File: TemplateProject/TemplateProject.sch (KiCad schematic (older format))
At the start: 0 parts

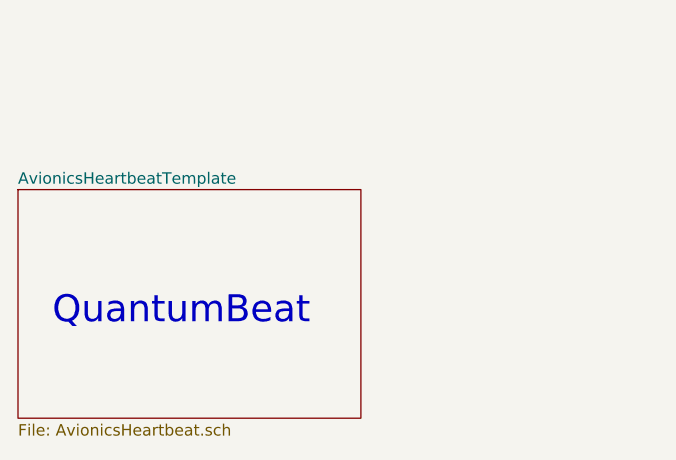
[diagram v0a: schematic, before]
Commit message: Rearrange QuantumBeat
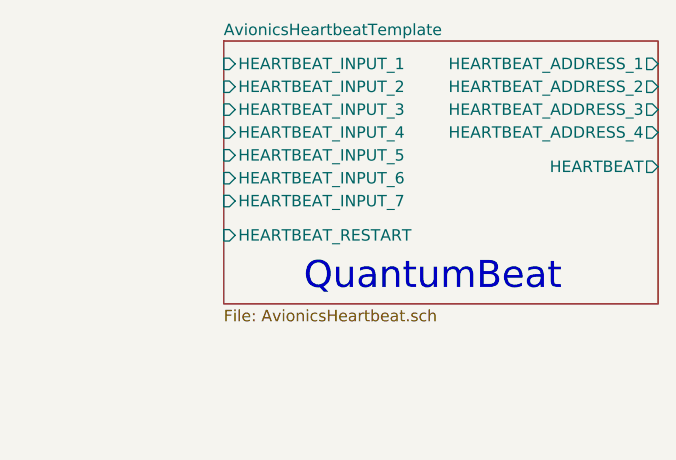
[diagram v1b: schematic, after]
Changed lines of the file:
@@
 $EndDescr
 $Sheet
-S 1500 1500 1500 1000
+S 2400 850  1900 1150
 U 5F94F01A
 F0 "AvionicsHeartbeatTemplate" 50
 F1 "AvionicsHeartbeat.sch" 50
+F2 "HEARTBEAT_INPUT_1" I L 2400 950 50
+F3 "HEARTBEAT_INPUT_2" I L 2400 1050 50
+F4 "HEARTBEAT_INPUT_3" I L 2400 1150 50
+F5 "HEARTBEAT_INPUT_4" I L 2400 1250 50
+F6 "HEARTBEAT_INPUT_5" I L 2400 1350 50
+F7 "HEARTBEAT_INPUT_6" I L 2400 1450 50
+F8 "HEARTBEAT_INPUT_7" I L 2400 1550 50
+F9 "HEARTBEAT_ADDRESS_1" O R 4300 950 50
+F10 "HEARTBEAT_ADDRESS_2" O R 4300 1050 50
+F11 "HEARTBEAT_ADDRESS_3" O R 4300 1150 50
+F12 "HEARTBEAT_ADDRESS_4" O R 4300 1250 50
+F13 "HEARTBEAT" O R 4300 1400 50
+F14 "HEARTBEAT_RESTART" I L 2400 1700 50
 $EndSheet
-Text Notes 1650 2100 0    118  ~ 0
+Text Notes 2750 1950 0    118  ~ 0
 QuantumBeat
 $EndSCHEMATC
